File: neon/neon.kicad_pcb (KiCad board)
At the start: 2 copper layers, 60 x 50 mm, 31 parts, among them J1 V3V3-VIO, J2 V3V3-GND, J3 V3V3-GND, J4 V3V3-GND, J5 VBUS-VCC, U1 FT4232H_module, U2 A, U3 B, U4 C, U5 D, U6 74HC595

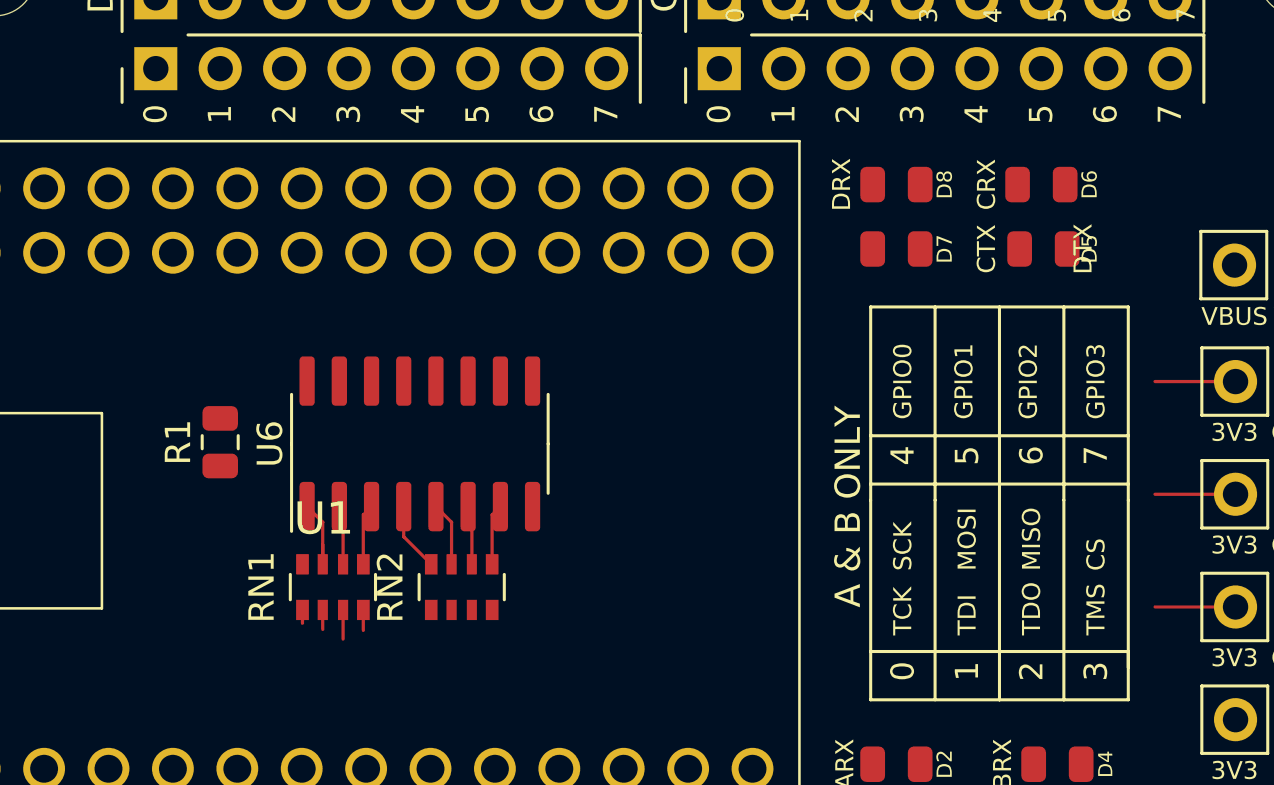
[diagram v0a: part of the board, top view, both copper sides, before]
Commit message: Fixes
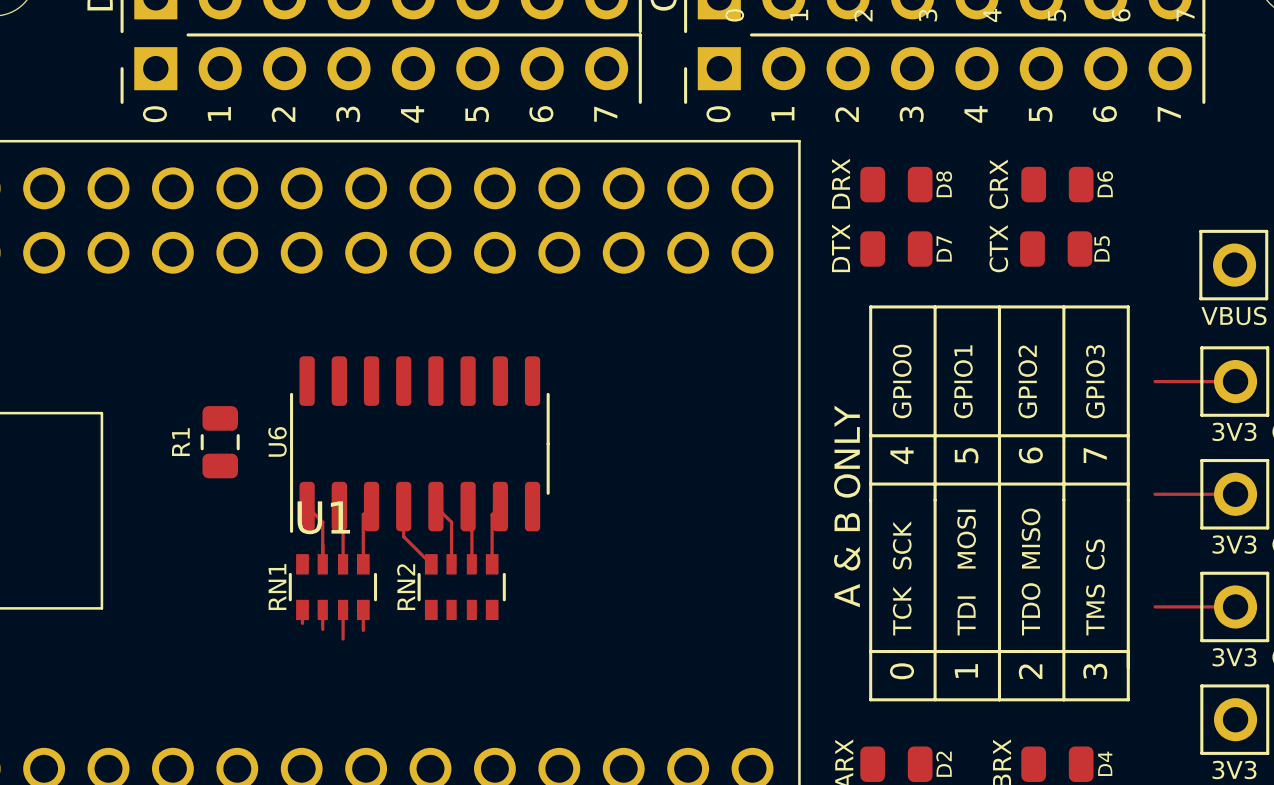
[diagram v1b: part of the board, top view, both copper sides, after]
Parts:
- moved D6 0.63 mm to (161.3, 92.1)
- moved D5 0.51 mm to (161.2, 94.6)
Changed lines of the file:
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@@
     (tags "resistor array")
     (attr smd)
-    (fp_text reference RN1 (at 0 -2.8 90) (layer F.SilkS)
-      (effects (font (size 1 1) (thickness 0.15)))
+    (fp_text reference RN1 (at 0 -2.159 90) (layer F.SilkS)
+      (effects (font (size 0.7 0.7) (thickness 0.15)))
     )
     (fp_text value 330 (at 0 2.8 90) (layer F.Fab)
@@
     (tags "resistor array")
     (attr smd)
-    (fp_text reference RN2 (at 0 -2.8 90) (layer F.SilkS)
-      (effects (font (size 1 1) (thickness 0.15)))
+    (fp_text reference RN2 (at 0 -2.159 90) (layer F.SilkS)
+      (effects (font (size 0.7 0.7) (thickness 0.15)))
     )
     (fp_text value 330 (at 0 2.8 90) (layer F.Fab)
@@
   )
   (module neon_footprints:LED_0805_2012Metric (layer F.Cu)
-    (at 160.655 92.075 180)
+    (at 161.29 92.075 180)
     (descr "LED SMD 0805 (2012 Metric), square (rectangular) end terminal, IPC_7351 nominal, (Body size source: https://docs.google.com/spreadsheets/d/1BsfQQcO9C6DZCsRaXUlFlo91Tg2WpOkGARC1WS5S8t0/edit?usp=sharing), generated with kicad-footprint-generator")
     (tags diode)
@@
   )
   (module neon_footprints:LED_0805_2012Metric (layer F.Cu)
-    (at 160.735 94.615 180)
+    (at 161.243 94.615 180)
     (descr "LED SMD 0805 (2012 Metric), square (rectangular) end terminal, IPC_7351 nominal, (Body size source: https://docs.google.com/spreadsheets/d/1BsfQQcO9C6DZCsRaXUlFlo91Tg2WpOkGARC1WS5S8t0/edit?usp=sharing), generated with kicad-footprint-generator")
     (tags diode)
@@
     (tags "SOIC SO")
     (attr smd)
-    (fp_text reference U6 (at 0 -5.9 90) (layer F.SilkS)
-      (effects (font (size 1 1) (thickness 0.15)))
+    (fp_text reference U6 (at 0.065 -5.588 90) (layer F.SilkS)
+      (effects (font (size 0.7 0.7) (thickness 0.15)))
     )
     (fp_text value 74HC595 (at 0 5.9 90) (layer F.Fab)
@@
     (tags resistor)
     (attr smd)
-    (fp_text reference R1 (at 0 -1.65 90) (layer F.SilkS)
-      (effects (font (size 1 1) (thickness 0.15)))
+    (fp_text reference R1 (at 0 -1.524 90) (layer F.SilkS)
+      (effects (font (size 0.7 0.7) (thickness 0.15)))
     )
     (fp_text value 10k (at 0 1.65 90) (layer F.Fab)
@@
     (effects (font (size 0.7112 0.7112) (thickness 0.175)))
   )
-  (gr_text CRX (at 158.496 92.075 90) (layer F.SilkS)
+  (gr_text CRX (at 159.004 92.075 90) (layer F.SilkS)
     (effects (font (size 0.7112 0.7112) (thickness 0.175)))
   )
@@
     (effects (font (size 0.7112 0.7112) (thickness 0.175)))
   )
-  (gr_text DTX (at 162.306 94.615 90) (layer F.SilkS)
+  (gr_text DTX (at 152.781 94.615 90) (layer F.SilkS)
     (effects (font (size 0.7112 0.7112) (thickness 0.175)))
   )
-  (gr_text CTX (at 158.496 94.615 90) (layer F.SilkS)
+  (gr_text CTX (at 159.004 94.615 90) (layer F.SilkS)
     (effects (font (size 0.7112 0.7112) (thickness 0.175)))
   )
